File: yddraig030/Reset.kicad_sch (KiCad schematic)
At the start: 18 parts, among them J201 ExtReset, J202 Ext RUN LED, Q201 BC858, Q202 BC858, SW201 Reset, U201 NE555P

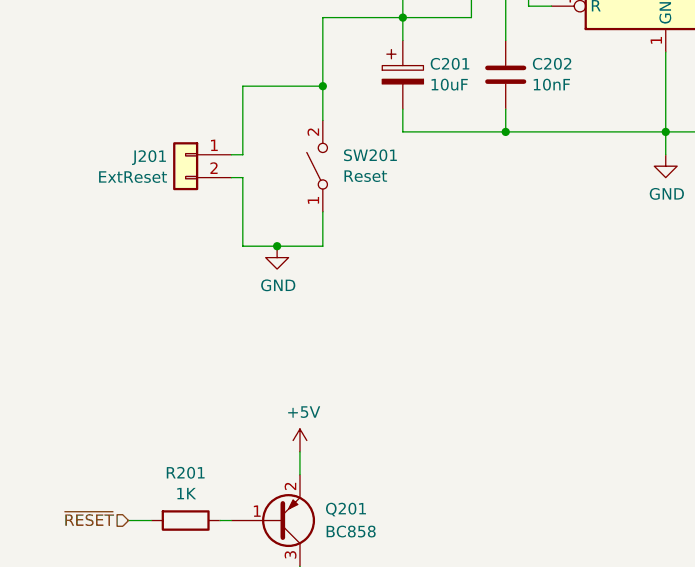
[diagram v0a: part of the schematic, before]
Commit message: Cleaning up schematic and PCB
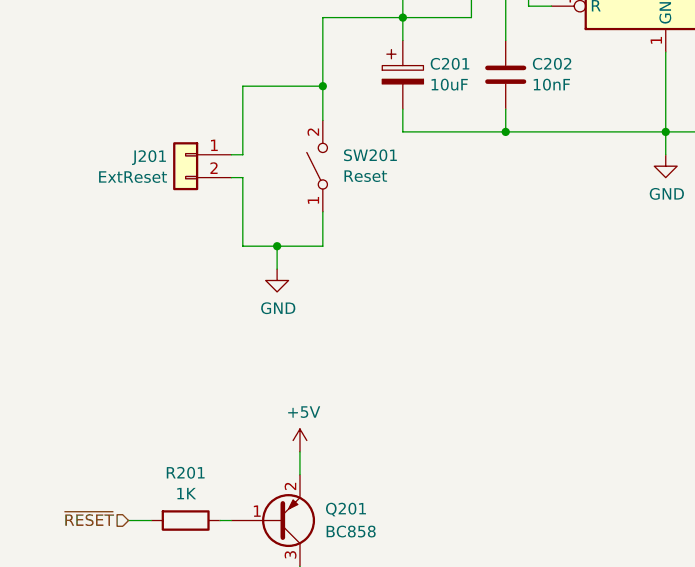
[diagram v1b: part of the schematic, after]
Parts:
- U201: footprint Package_SO:SO-8_5.3x6.2mm_P1.27mm -> Package_SO:SOIC-8_3.9x4.9mm_P1.27mm
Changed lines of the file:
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@@
+    (stroke (width 0) (type default) (color 0 0 0 0))
+  )
+  (wire (pts (xy 92.71 90.17) (xy 97.79 90.17))
     (stroke (width 0) (type default) (color 0 0 0 0))
   )
@@
     (stroke (width 0) (type default) (color 0 0 0 0))
   )
+  (wire (pts (xy 114.3 64.77) (xy 106.68 64.77))
+    (stroke (width 0) (type default) (color 0 0 0 0))
+  )
+  (wire (pts (xy 118.11 77.47) (xy 106.68 77.47))
+    (stroke (width 0) (type default) (color 0 0 0 0))
+  )
+  (wire (pts (xy 76.2 120.65) (xy 78.74 120.65))
+    (stroke (width 0) (type default) (color 0 0 0 0))
+  )
+  (wire (pts (xy 135.89 77.47) (xy 135.89 80.01))
+    (stroke (width 0) (type default) (color 0 0 0 0))
+  )
   (wire (pts (xy 88.9 90.17) (xy 92.71 90.17))
     (stroke (width 0) (type default) (color 0 0 0 0))
   )
-  (wire (pts (xy 114.3 64.77) (xy 106.68 64.77))
-    (stroke (width 0) (type default) (color 0 0 0 0))
-  )
-  (wire (pts (xy 118.11 77.47) (xy 106.68 77.47))
-    (stroke (width 0) (type default) (color 0 0 0 0))
-  )
-  (wire (pts (xy 76.2 120.65) (xy 78.74 120.65))
-    (stroke (width 0) (type default) (color 0 0 0 0))
-  )
-  (wire (pts (xy 135.89 77.47) (xy 135.89 80.01))
-    (stroke (width 0) (type default) (color 0 0 0 0))
-  )
-  (wire (pts (xy 97.79 90.17) (xy 92.71 90.17))
-    (stroke (width 0) (type default) (color 0 0 0 0))
-  )
   (wire (pts (xy 135.89 77.47) (xy 152.4 77.47))
     (stroke (width 0) (type default) (color 0 0 0 0))
@@
   )
   (wire (pts (xy 95.25 125.73) (xy 95.25 129.54))
+    (stroke (width 0) (type default) (color 0 0 0 0))
+  )
+  (wire (pts (xy 92.71 90.17) (xy 92.71 92.71))
     (stroke (width 0) (type default) (color 0 0 0 0))
   )
@@
     (property "Reference" "U201" (id 0) (at 130.81 48.26 0))
     (property "Value" "NE555P" (id 1) (at 140.97 48.26 0))
-    (property "Footprint" "Package_SO:SO-8_5.3x6.2mm_P1.27mm" (id 2) (at 152.4 68.58 0)
+    (property "Footprint" "Package_SO:SOIC-8_3.9x4.9mm_P1.27mm" (id 2) (at 152.4 68.58 0)
       (effects (font (size 1.27 1.27)) hide)
     )
@@
     (pin "1")
   )
-  (symbol (lib_id "power:GND") (at 92.71 90.17 0) (unit 1)
-    (in_bom yes) (on_board yes)
-    (property "Reference" "#PWR0201" (id 0) (at 92.71 96.52 0)
-      (effects (font (size 1.27 1.27)) hide)
-    )
-    (property "Value" "GND" (id 1) (at 92.837 94.5642 0))
-    (property "Footprint" "" (id 2) (at 92.71 90.17 0)
-      (effects (font (size 1.27 1.27)) hide)
-    )
-    (property "Datasheet" "" (id 3) (at 92.71 90.17 0)
-      (effects (font (size 1.27 1.27)) hide)
-    )
+  (symbol (lib_id "power:GND") (at 92.71 92.71 0) (unit 1)
+    (in_bom yes) (on_board yes)
+    (property "Reference" "#PWR0201" (id 0) (at 92.71 99.06 0)
+      (effects (font (size 1.27 1.27)) hide)
+    )
+    (property "Value" "GND" (id 1) (at 92.837 97.1042 0))
+    (property "Footprint" "" (id 2) (at 92.71 92.71 0)
+      (effects (font (size 1.27 1.27)) hide)
+    )
+    (property "Datasheet" "" (id 3) (at 92.71 92.71 0)
+      (effects (font (size 1.27 1.27)) hide)
+    )
